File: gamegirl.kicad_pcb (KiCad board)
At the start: 2 copper layers, 175 x 70 mm, 58 parts, among them J1 Conn_01x07_Socket, J2 Conn_01x14_Socket, J3 Conn_01x04_Socket, SW1 EN, SW10 select, SW12 SS12D07VG4 087, SW2 up, SW3 down, SW4 left, SW5 right, SW6 A, SW7 B, SW9 start, U1 ESP32-WROOM-32, U2 AP2112K-3.3, U3 CH340N_C2977777

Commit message: traces of doom and despair
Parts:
- SW12: moved to F.Cu
- moved SW12 218.6 mm to (17.0, 8.75), turned to -90 degrees
- moved J1 200.8 mm to (25.2, 3.17)
- moved D2 108.6 mm to (140.2, 11.5)
- moved R16 108.6 mm to (134.7, 11.8)
- moved SW7 106.8 mm to (143.5, 23.8)
- moved H8 104.9 mm to (120.2, 57.2)
- moved SW9 104.2 mm to (143.5, 42.0)
- moved J3 103.1 mm to (120.2, 31.4)
- moved C10 100.4 mm to (145.4, 51.7)
- moved C11 100.4 mm to (138.8, 69.5)
- moved C12 100.4 mm to (130.7, 59.8)
- moved R15 100.4 mm to (130.3, 66.4)
- moved H4 99.5 mm to (153.5, 64.0)
- moved H7 99.4 mm to (120.2, 13.2)
- moved SW6 99.4 mm to (131.5, 31.0)
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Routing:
- net VBUS: track 130.9 -> 21.0 mm, vias 1 -> 0
- net /left: track 101.0 -> 10.3 mm, vias 2 -> 0
- net /select: track 88.1 -> 0.00 mm, vias 1 -> 0
- net /GPIO22: track 85.7 -> 0.00 mm, vias 1 -> 0
- net /down: track 86.4 -> 2.21 mm, vias 3 -> 0
- net /status: track 91.6 -> 7.45 mm, vias 3 -> 1
- net /start: track 83.1 -> 0.00 mm
- net /GPIO26: track 60.6 -> 0.00 mm, vias 1 -> 0
- net /GPIO25: track 61.5 -> 2.41 mm
- net /right: track 73.2 -> 23.2 mm, vias 2 -> 1
- net /up: track 45.2 -> 1.99 mm
- net /GPIO14: track 61.4 -> 35.1 mm
- net /GPIO15: track 72.7 -> 49.0 mm
- net GND: track 59.6 -> 36.2 mm
- net /GPIO12: track 58.6 -> 37.9 mm
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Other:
- board size 175 x 70 mm -> 160 x 70 mm

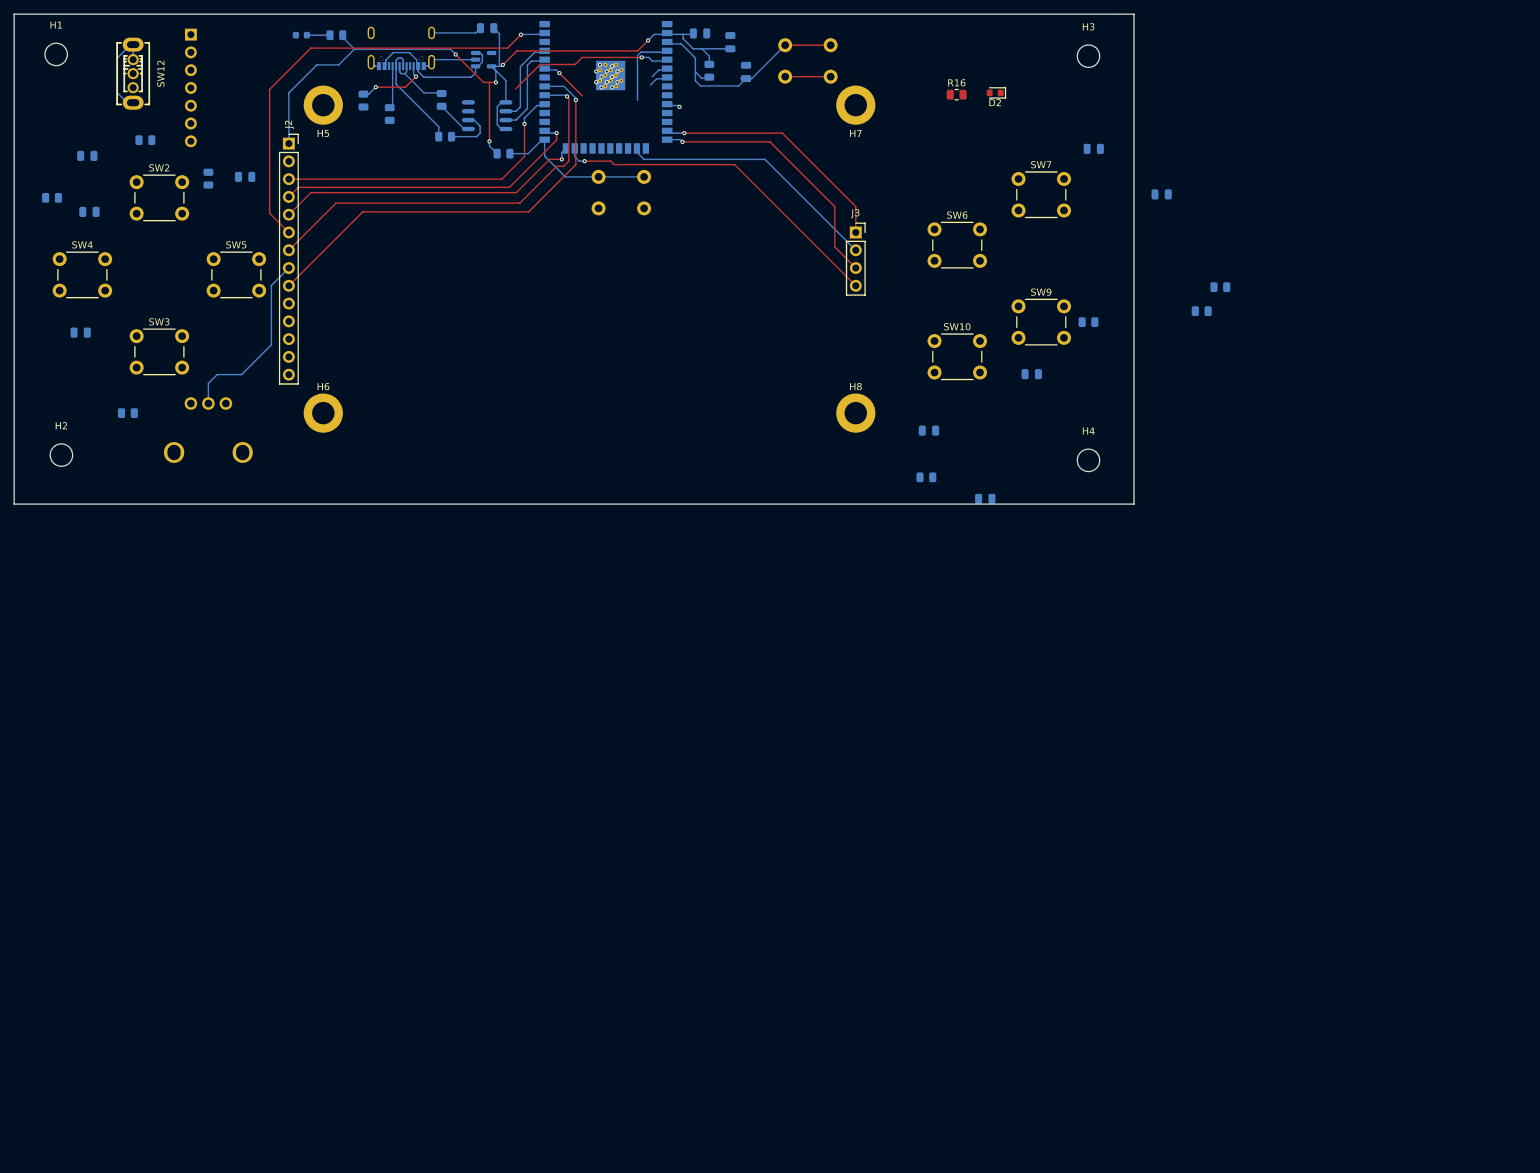
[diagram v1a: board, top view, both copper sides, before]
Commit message: final? layout
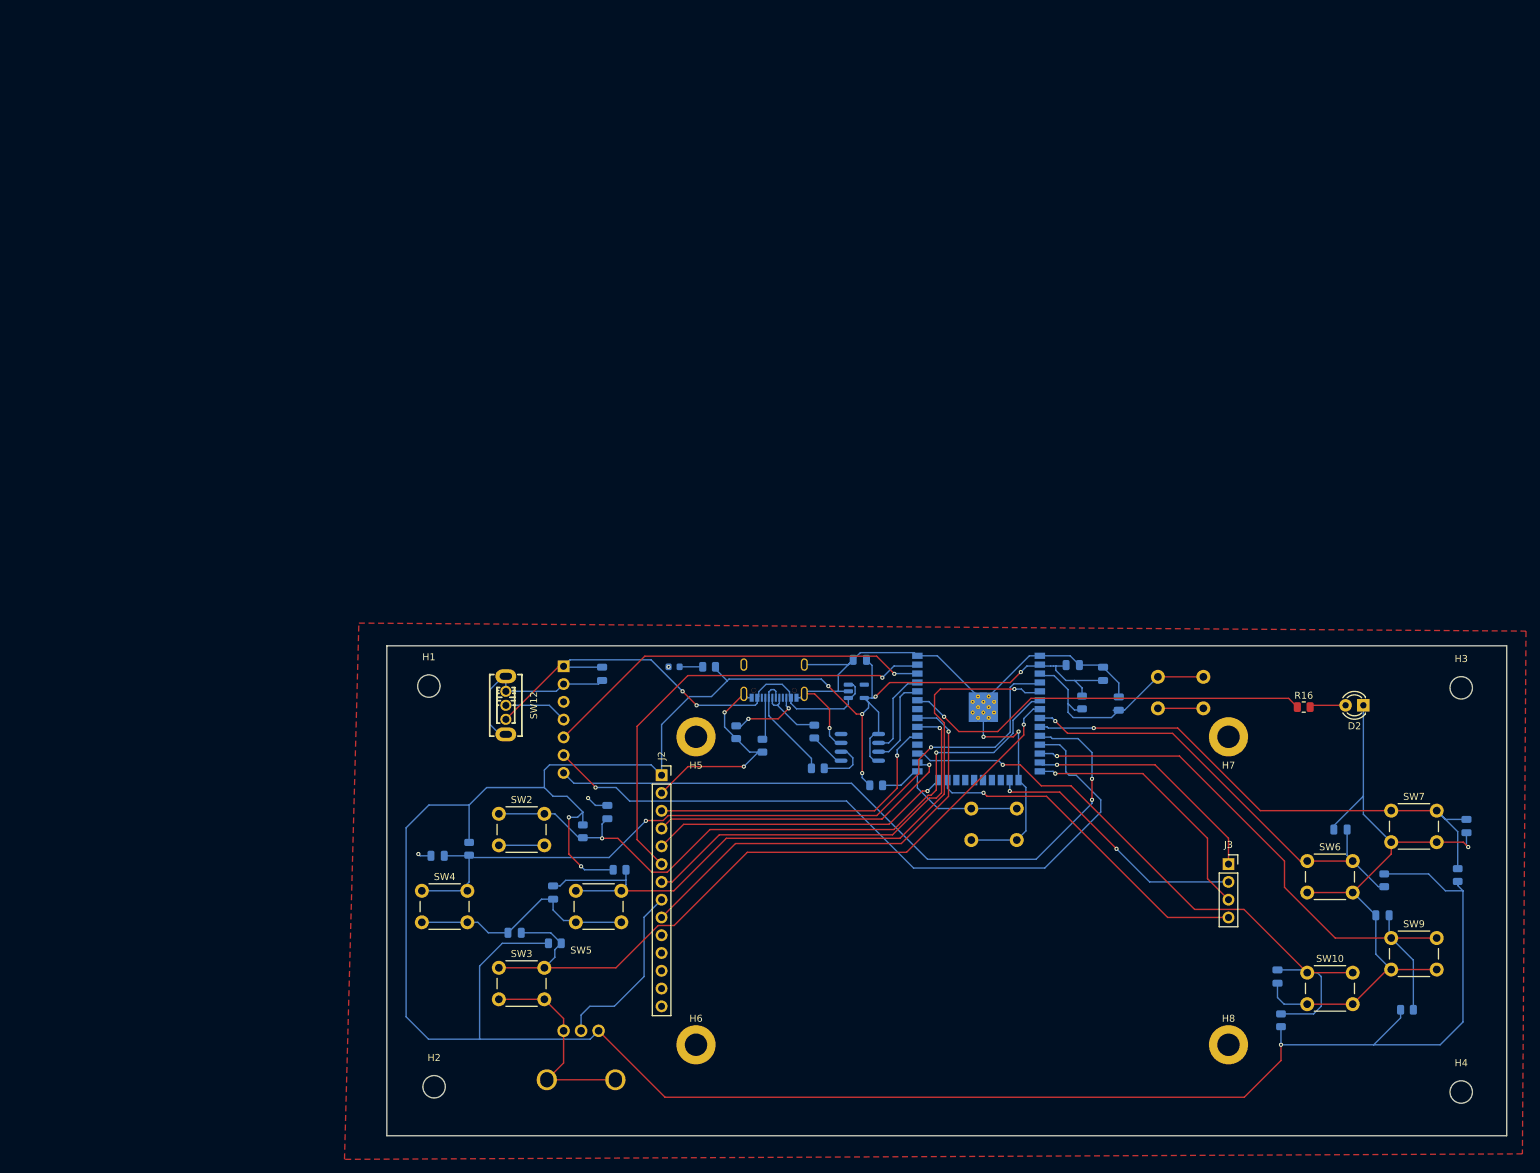
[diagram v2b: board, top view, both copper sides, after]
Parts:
- D2: footprint LED_SMD:LED_0603_1608Metric -> LED_THT:LED_D3.0mm
- moved C5 119.6 mm to (84.8, 114.2), turned to 90 degrees
- moved R7 116.9 mm to (81.2, 117.0), turned to 90 degrees
- moved R10 114.9 mm to (86.5, 122.5), turned to 180 degrees
- moved C8 111.3 mm to (77.0, 125.8), turned to -90 degrees
- moved R9 110.5 mm to (65.0, 119.5), turned to 90 degrees
- moved R14 108.3 mm to (199.0, 142.5), turned to 180 degrees
- moved C6 105.8 mm to (71.5, 131.5)
- moved C13 105.3 mm to (84.0, 94.5), turned to -90 degrees
- moved BOOT 104.8 mm to (143.2, 113.8)
- moved C1 104.8 mm to (120.8, 92.5)
- moved C4 104.8 mm to (151.2, 93.2)
- moved D1 104.8 mm to (94.3, 93.5)
- moved H1 104.8 mm to (59.2, 96.2)
- moved H2 104.8 mm to (60.0, 153.5)
- moved H3 104.8 mm to (206.8, 96.5)
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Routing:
- net +3V3: track 116.1 -> 440.0 mm, vias 5 -> 8
- net GND: track 36.2 -> 345.2 mm, vias 12 -> 9
- net /down: track 2.21 -> 104.8 mm, vias 0 -> 1
- net /GPIO26: track 0.00 -> 102.3 mm, vias 0 -> 1
- net /left: track 10.3 -> 110.8 mm, vias 0 -> 2
- net /GPIO25: track 2.41 -> 100.1 mm, vias 1 -> 2
- net /up: track 1.99 -> 97.6 mm, vias 0 -> 2
- net /select: track 0.00 -> 92.3 mm, vias 0 -> 1
- net /start: track 0.00 -> 84.8 mm, vias 0 -> 1
- net /right: track 23.2 -> 102.6 mm
- net /B: track 0.00 -> 76.0 mm, vias 0 -> 1
- net /A: track 0.00 -> 64.0 mm, vias 0 -> 1
- net /GPIO22: track 0.00 -> 56.4 mm, vias 0 -> 1
- net /status: track 7.45 -> 59.1 mm
- net VBUS: track 21.0 -> 69.6 mm, vias 0 -> 2
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- added copper zone on F.Cu, net GND
